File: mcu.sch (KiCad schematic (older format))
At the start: 18 parts, among them SW19 EVQQ2, SW8 EVQQ2, U9 STM32F405RGTx, Y1 8MHz

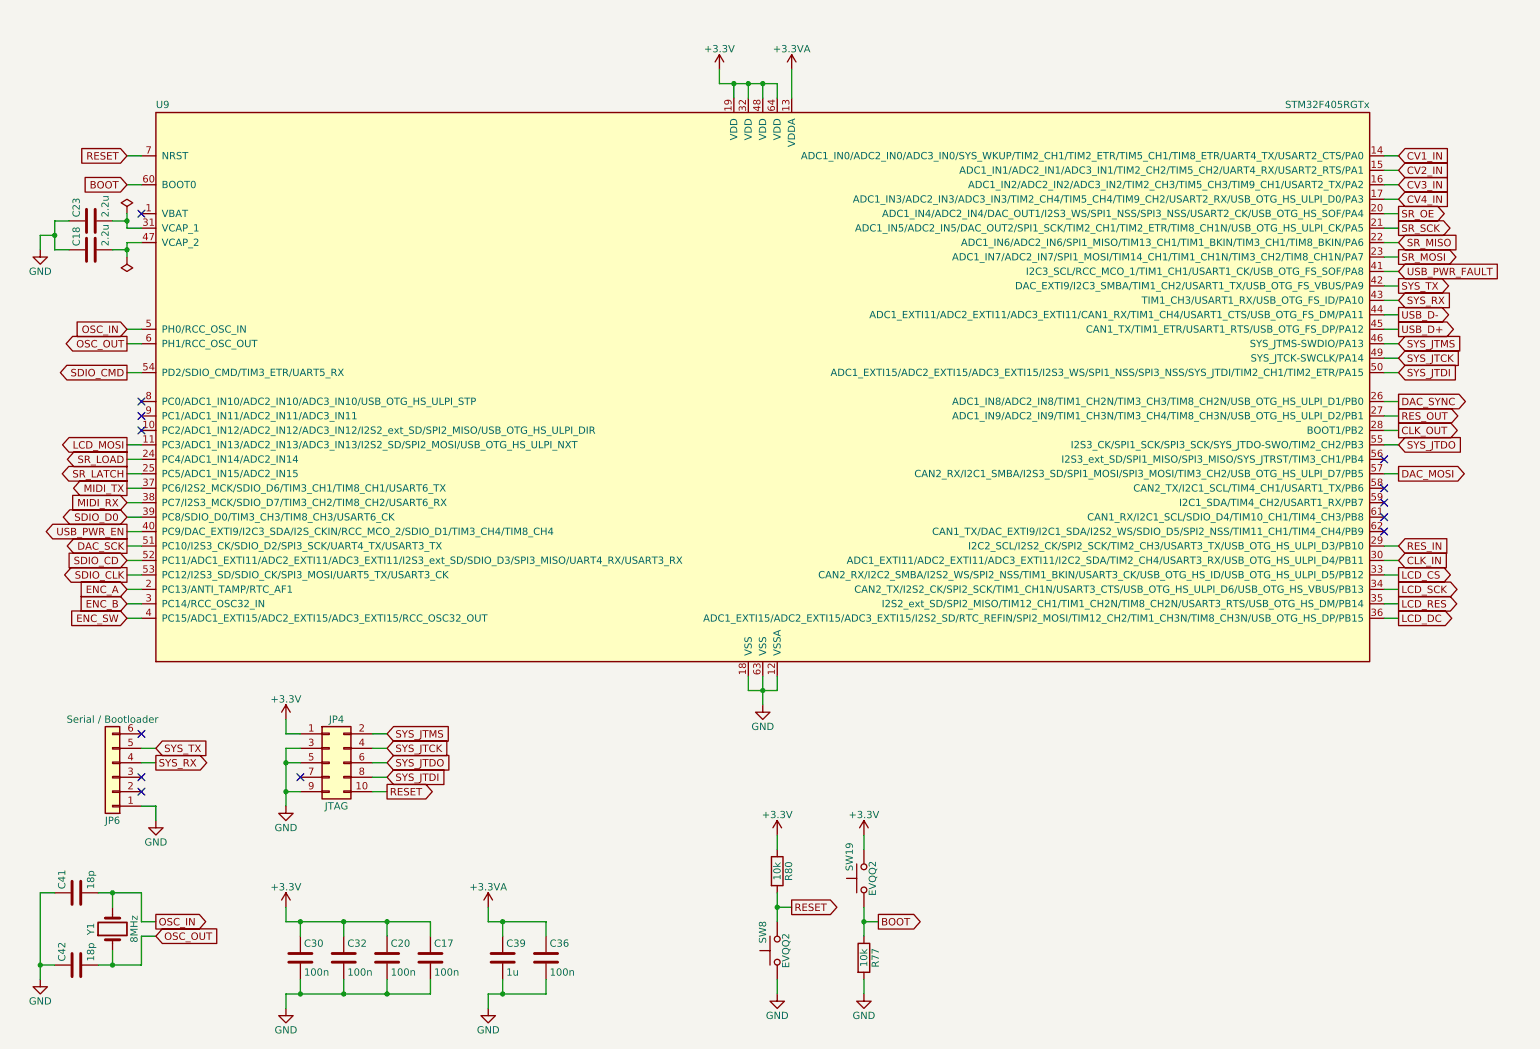
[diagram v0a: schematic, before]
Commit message: cleaned up schematics
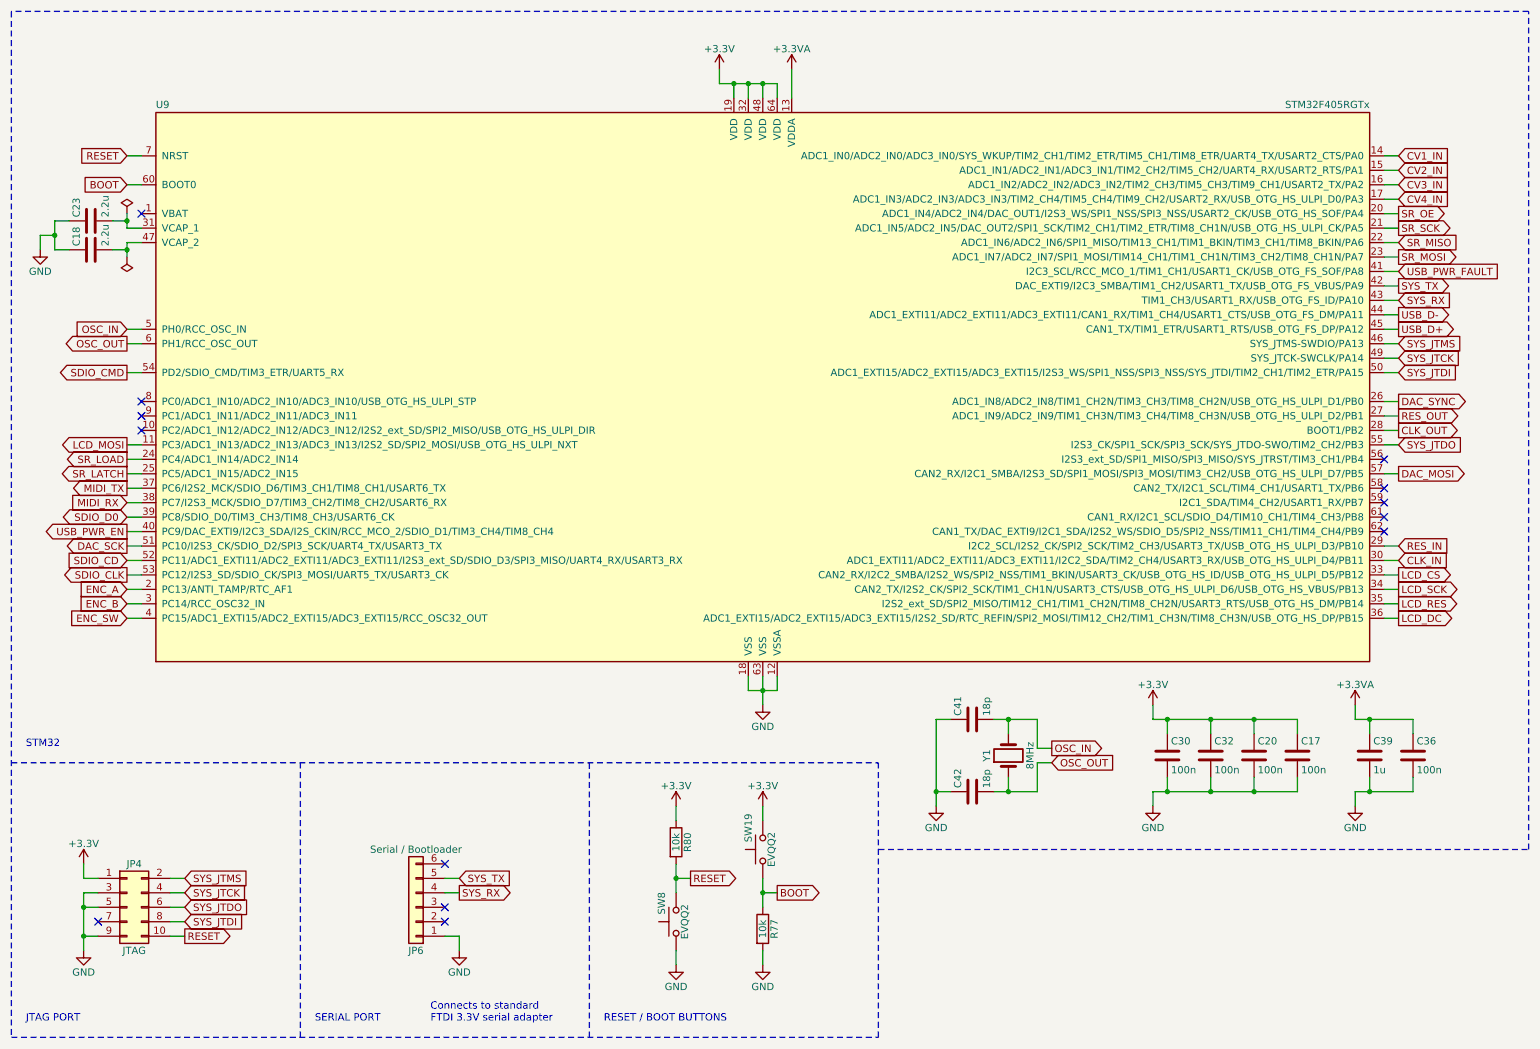
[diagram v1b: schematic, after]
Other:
- note added: "Connects to standard\nFTDI 3.3V serial adapter"
- note added: "JTAG PORT"
- note added: "RESET / BOOT BUTTONS"
- note added: "SERIAL PORT"
- note added: "STM32"
- moved on the sheet: C17, C20, C30, C32, C36, C39, C41, C42, JP4, JP6, R77, R80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
